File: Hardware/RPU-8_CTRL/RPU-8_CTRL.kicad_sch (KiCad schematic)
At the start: 8 parts, among them J1 ADDR_BUS, J2 DATA_BUS, J3 Conn_01x03_Female, J4 CTRL_BUS, U1 AT28C16, U2 AT28C16, U3 AT28C16

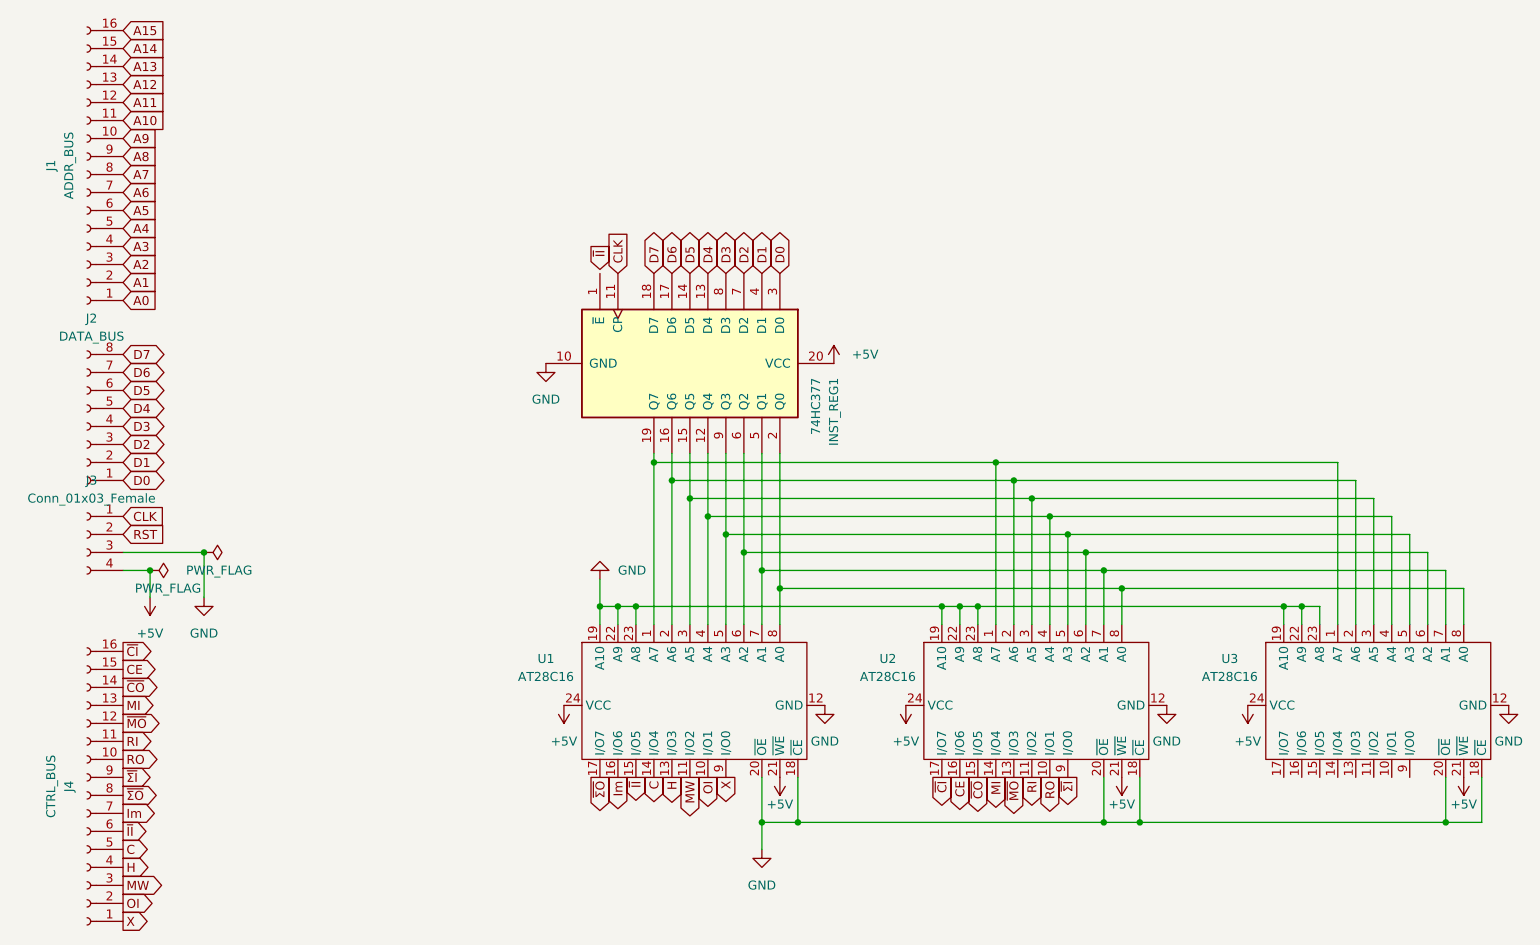
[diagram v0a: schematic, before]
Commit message: add .readthedocs.yaml
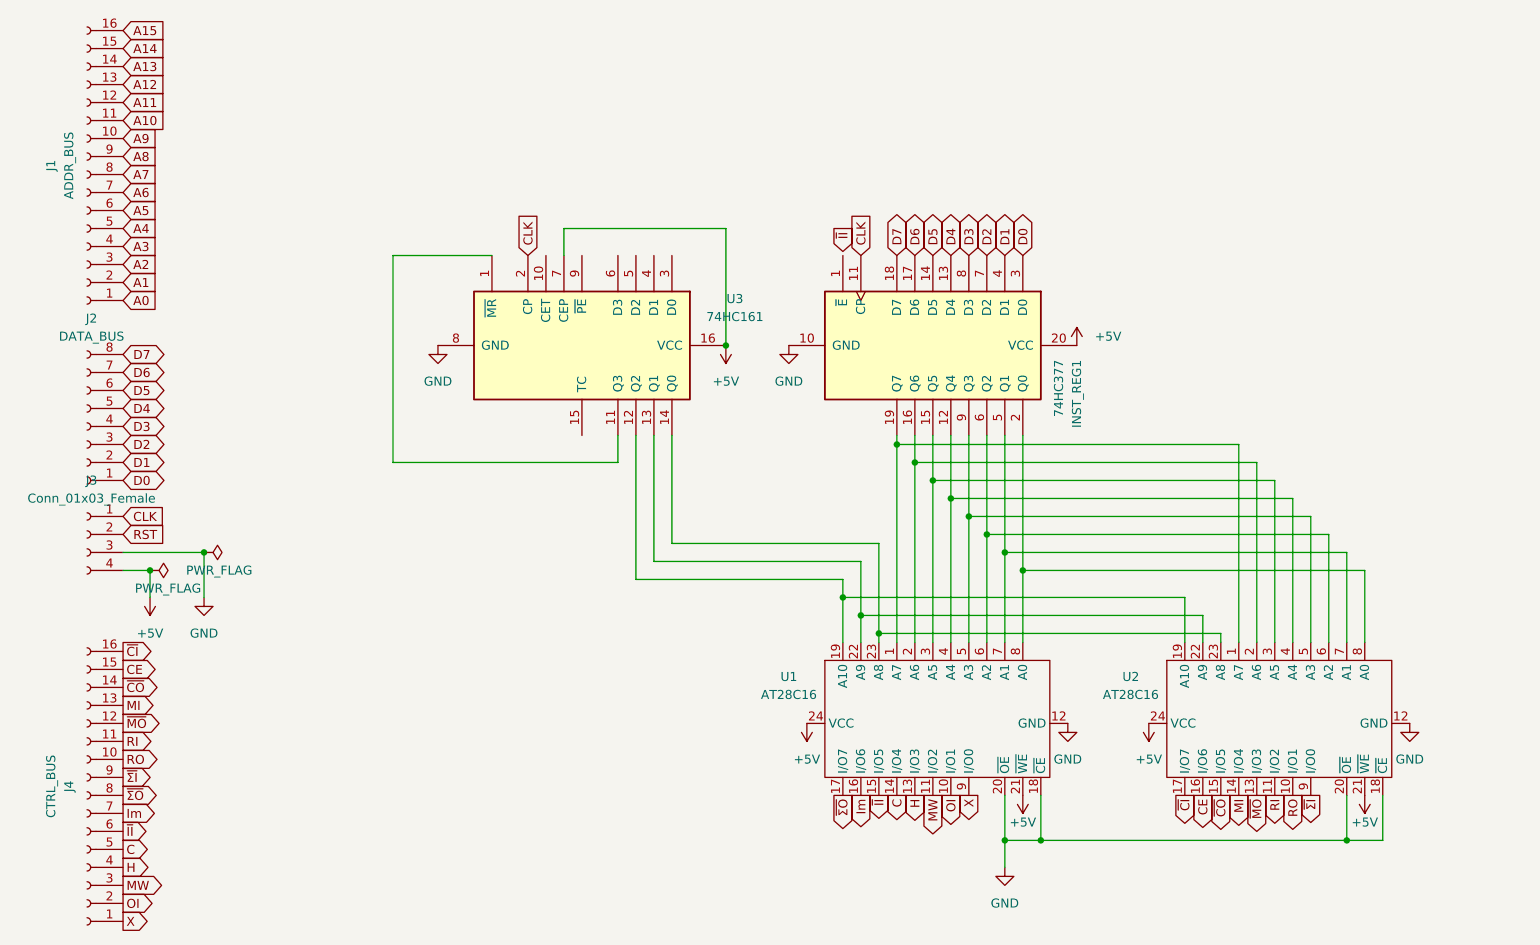
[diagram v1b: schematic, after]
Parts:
- removed U3: AT28C16, Package_DIP:DIP-24_W15.24mm_Socket, symbol Memory_EEPROM:AT28C16
- added U3: 74HC161, Package_DIP:DIP-16_W7.62mm_Socket, symbol 74xx:74HC161
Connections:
- net +5V: now also U3.16 (VCC), U3.7 (CEP)
- net CLK: now also U3.2 (CP)
- net GND: now also U3.8 (GND); no longer U1.19 (A10), U1.22 (A9), U1.23 (A8), U2.19 (A10), U2.22 (A9), U2.23 (A8)
- new net: U1.19 (A10), U2.19 (A10), U3.12 (Q2)
- new net: U1.22 (A9), U2.22 (A9), U3.13 (Q1)
- new net: U1.23 (A8), U2.23 (A8), U3.14 (Q0)
- new net: U3.1 (~{MR}), U3.11 (Q3)
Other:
- moved on the sheet: INST_REG1, U1, U2
